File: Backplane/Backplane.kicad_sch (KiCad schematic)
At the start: 0 parts

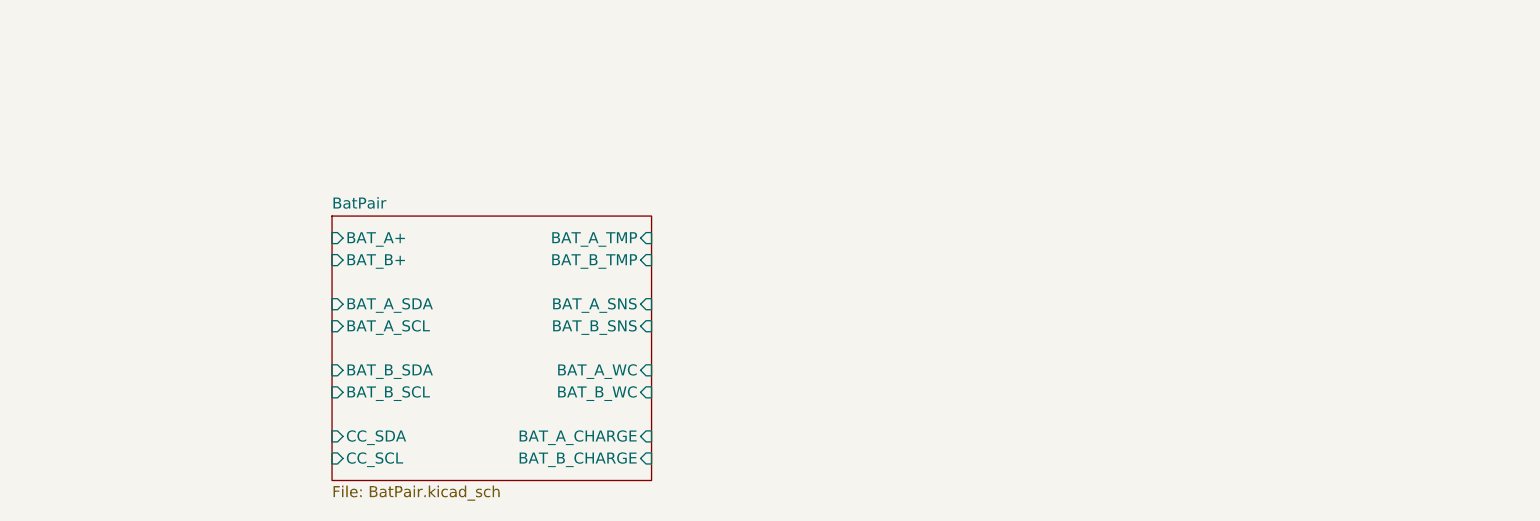
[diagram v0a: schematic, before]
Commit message: Working on Analog Section.
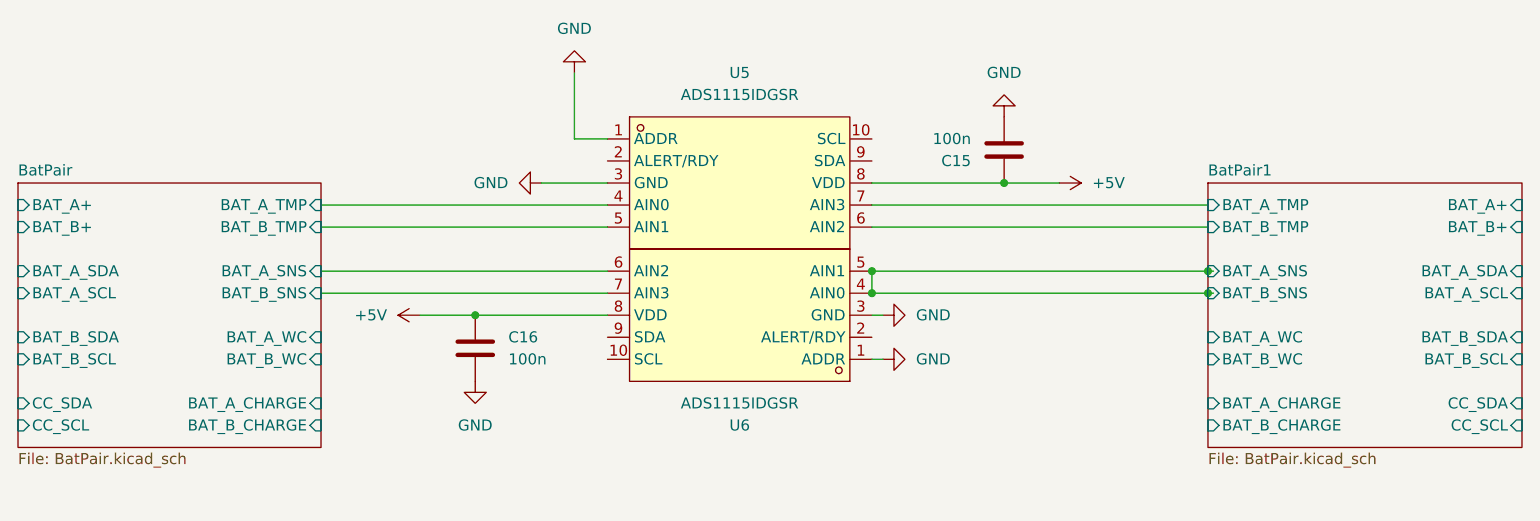
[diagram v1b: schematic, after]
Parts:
- added C15, C16: 100n, Resistor_SMD:R_1206_3216Metric_Pad1.30x1.75mm_HandSolder, symbol Device:C
- added U5, U6: ADS1115IDGSR, COMPONENTS:MSOP-10_L3.0-W3.0-P0.50-LS5.0-BL, symbol COMPONENTS:ADS1115IDGSR
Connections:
- net BatPair/BAT_A_SNS: now also U6.6 (AIN2)
- net BatPair/BAT_A_TMP: now also U5.4 (AIN0)
- net BatPair/BAT_B_SNS: now also U6.7 (AIN3)
- net BatPair/BAT_B_TMP: now also U5.5 (AIN1)
- new net +5V: C15.1, C16.1, U5.8 (VDD), U6.8 (VDD)
- new net BatPair1/BAT_A_SNS: U6.4 (AIN0), U6.5 (AIN1)
- new net BatPair1/BAT_A_TMP: U5.7 (AIN3)
- new net BatPair1/BAT_B_TMP: U5.6 (AIN2)
- new net GND: C15.2, C16.2, U5.1 (ADDR), U5.3 (GND), U6.1 (ADDR), U6.3 (GND)
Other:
- added sheet BatPair1 (BatPair.kicad_sch)
